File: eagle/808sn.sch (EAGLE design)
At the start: 75 parts, among them IC1 TL072P, IC3 TL072P, Q1 2N3904, Q45 2N3904, Q46 2N3906, Q47 2N3904, Q48 2N3904, Q49 2N3904, U1 POWER

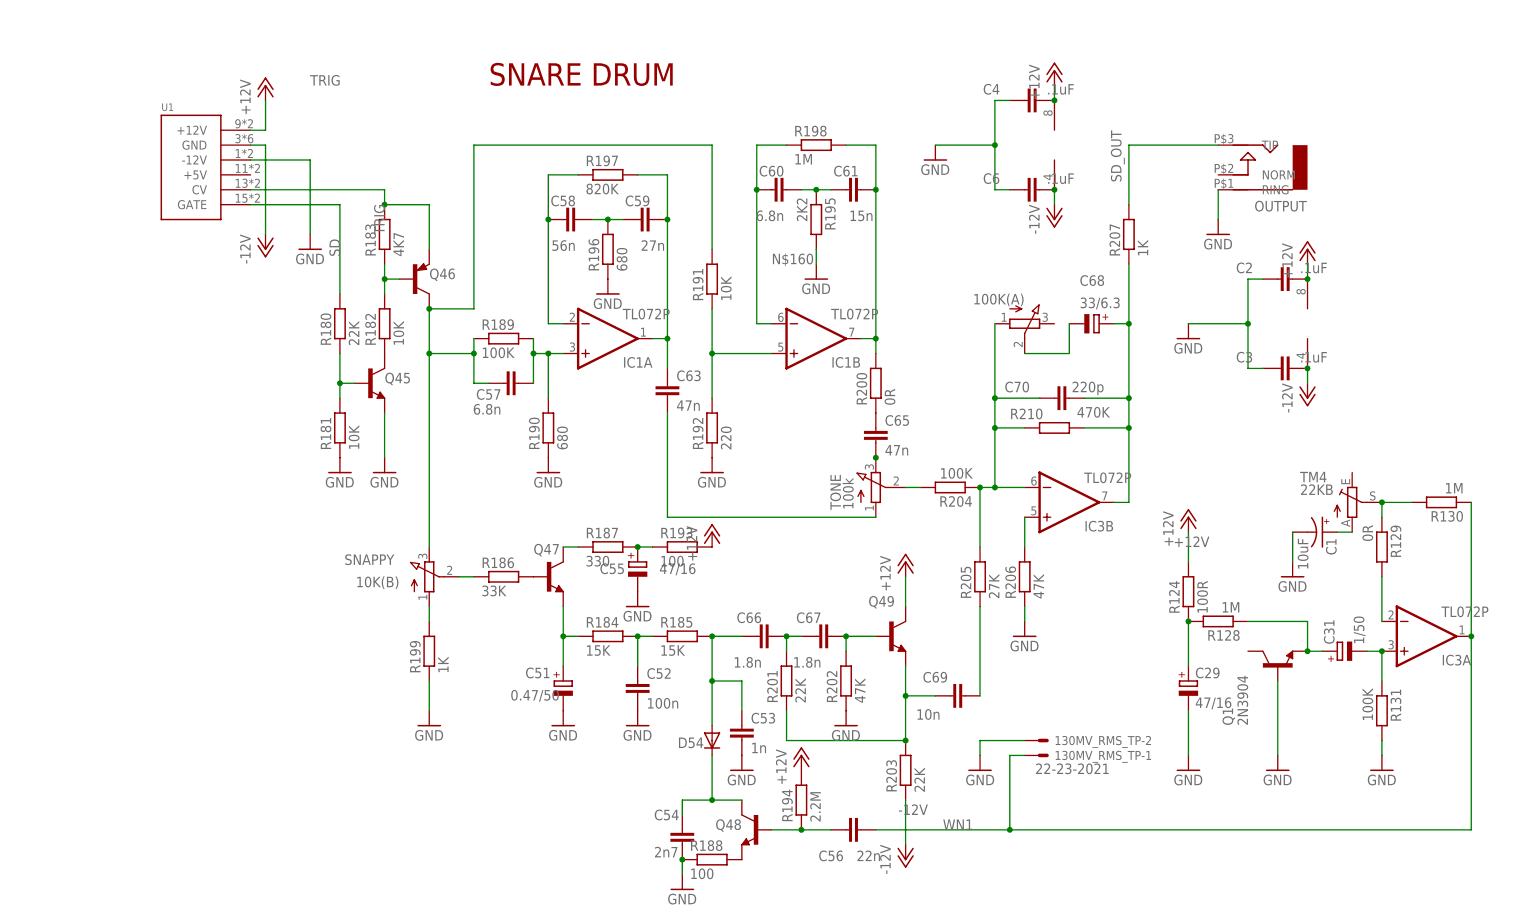
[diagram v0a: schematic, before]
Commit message: 92pct autorouted
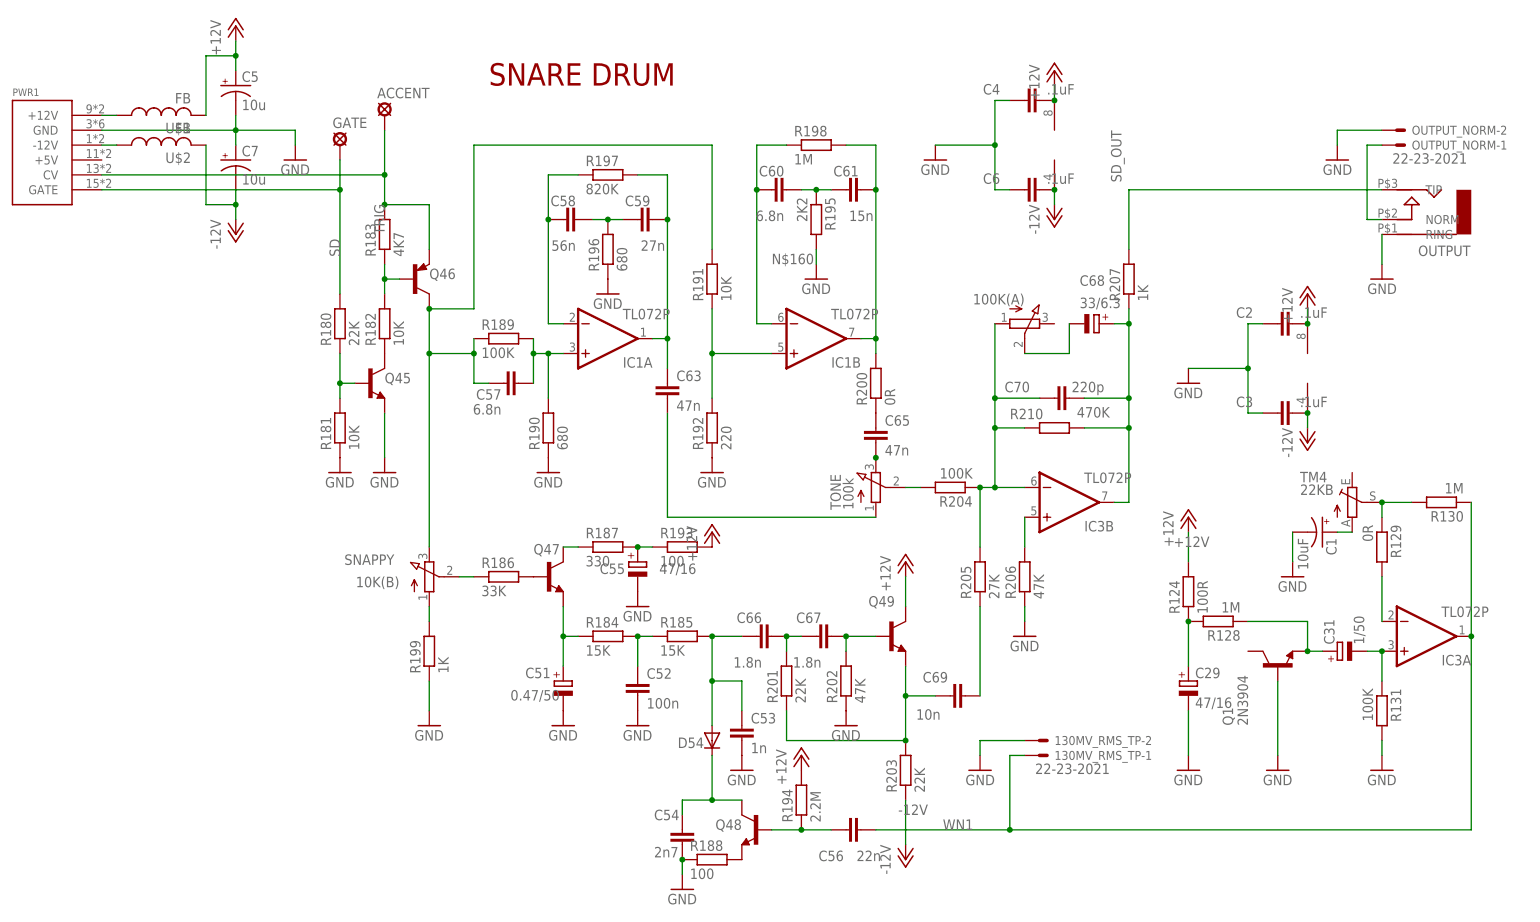
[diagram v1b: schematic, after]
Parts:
- removed U1: POWER, eurorack:POWER
- added ACCENT, GATE: LSP10, solpad:LSP10
- added C5, C7: 10u, rcl:CPOL-USB45181A
- added OUTPUT_NORM: 22-23-2021, con-molex:22-23-2021
- added PWR1: POWER, eurorack:POWER
- added U$1, U$2: FB, adafruit:FB
- R187, R193, R195, R196, R201, R205: device TR808clone:R-EU_0207/5V -> TR808clone:R-EU_0207/7
- R194, R203, R207: device TR808clone:R-EU_0207/5V -> TR808clone:R-EU_0309/10
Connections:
- new net N$10: PWR1.+12V, U$1.1
- new net N$2: OUTPUT.NORM, OUTPUT_NORM-1.S
- new net N$37: PWR1.-12V, U$2.1
- net +12V: now also C5.+, U$1.2; no longer U1.+12V
- net -12V: now also C7.-, U$2.2; no longer U1.GND
- net GND: now also OUTPUT_NORM-2.S; no longer U1.-12V
- net N$26: now also C5.-, C7.+, PWR1.GND
- net SD: now also GATE.MP, PWR1.GATE; no longer U1.GATE
- net TRIG: now also ACCENT.MP, PWR1.CV; no longer U1.CV
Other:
- moved on the sheet: C2, C3, OUTPUT, R207

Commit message: board started over
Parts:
- C52: device TR808clone:C-EU075-032X103 -> TR808clone:C-EU050-045X075
- C6: device TR808clone:C-EU025-025X050 -> TR808clone:C-EU050-025X075
- C69: device TR808clone:C-EU3.5MM_PITCH -> TR808clone:C-EU075-042X103
- R194, R203: device TR808clone:R-EU_0309/10 -> TR808clone:R-EU_0207/7
- R204: device TR808clone:R-EU_0207/5V -> TR808clone:R-EU_0207/7
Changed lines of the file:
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@@
 <part name="R184" library="TR808clone" deviceset="R-EU_" device="0207/5V" value="15K"/>
 <part name="R185" library="TR808clone" deviceset="R-EU_" device="0207/5V" value="15K"/>
-<part name="C52" library="TR808clone" deviceset="C-EU" device="075-032X103" value="100n"/>
+<part name="C52" library="TR808clone" deviceset="C-EU" device="050-045X075" value="100n"/>
 <part name="C55" library="TR808clone" deviceset="CPOL-EU" device="E2-5" value="47/16"/>
 <part name="C51" library="TR808clone" deviceset="CPOL-EU" device="E2-5" value="0.47/50"/>
@@
 <part name="GND13" library="supply1" deviceset="GND" device=""/>
 <part name="GND14" library="supply1" deviceset="GND" device=""/>
-<part name="R203" library="TR808clone" deviceset="R-EU_" device="0309/10" value="22K"/>
+<part name="R203" library="TR808clone" deviceset="R-EU_" device="0207/7" value="22K"/>
 <part name="Q48" library="808_lt" deviceset="2N3904" device=""/>
 <part name="C54" library="TR808clone" deviceset="C-EU" device="3.5MM_PITCH" value="2n7"/>
 <part name="R188" library="TR808clone" deviceset="R-EU_" device="0207/5V" value="100"/>
-<part name="R194" library="TR808clone" deviceset="R-EU_" device="0309/10" value="2.2M"/>
+<part name="R194" library="TR808clone" deviceset="R-EU_" device="0207/7" value="2.2M"/>
 <part name="C56" library="TR808clone" deviceset="C-EU" device="4MM_PITCH" value="22n"/>
 <part name="GND58" library="supply1" deviceset="GND" device=""/>
-<part name="C69" library="TR808clone" deviceset="C-EU" device="3.5MM_PITCH" value="10n"/>
-<part name="R204" library="TR808clone" deviceset="R-EU_" device="0207/5V" value="100K"/>
+<part name="C69" library="TR808clone" deviceset="C-EU" device="075-042X103" value="10n"/>
+<part name="R204" library="TR808clone" deviceset="R-EU_" device="0207/7" value="100K"/>
 <part name="R205" library="TR808clone" deviceset="R-EU_" device="0207/7" value="27K"/>
 <part name="R206" library="TR808clone" deviceset="R-EU_" device="0207/5V" value="47K"/>
@@
 <part name="IC1" library="linear" deviceset="TL072" device="P"/>
 <part name="C4" library="TR808clone" deviceset="C-EU" device="025-025X050" value=".1uF"/>
-<part name="C6" library="TR808clone" deviceset="C-EU" device="025-025X050" value=".1uF"/>
+<part name="C6" library="TR808clone" deviceset="C-EU" device="050-025X075" value=".1uF"/>
 <part name="GND15" library="supply1" deviceset="GND" device=""/>
 <part name="R130" library="TR808clone" deviceset="R-EU_" device="0207/7" value="1M"/>

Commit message: 94pct autorouted
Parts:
- R183, R189: device TR808clone:R-EU_0207/5V -> TR808clone:R-EU_0207/2V
- R186: device TR808clone:R-EU_0207/5V -> TR808clone:R-EU_0309/12
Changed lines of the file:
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@@
 <part name="R181" library="TR808clone" deviceset="R-EU_" device="0207/5V" value="10K"/>
 <part name="R182" library="TR808clone" deviceset="R-EU_" device="0207/5V" value="10K"/>
-<part name="R183" library="TR808clone" deviceset="R-EU_" device="0207/5V" value="4K7"/>
+<part name="R183" library="TR808clone" deviceset="R-EU_" device="0207/2V" value="4K7"/>
 <part name="Q45" library="808_lt" deviceset="2N3904" device=""/>
 <part name="Q46" library="808_lt" deviceset="2N3906" device=""/>
@@
 <part name="C59" library="TR808clone" deviceset="C-EU" device="050-024X044" value="27n"/>
 <part name="C57" library="TR808clone" deviceset="C-EU" device="4MM_PITCH" value="6.8n"/>
-<part name="R189" library="TR808clone" deviceset="R-EU_" device="0207/5V" value="100K"/>
+<part name="R189" library="TR808clone" deviceset="R-EU_" device="0207/2V" value="100K"/>
 <part name="R196" library="TR808clone" deviceset="R-EU_" device="0207/7" value="680"/>
 <part name="R197" library="TR808clone" deviceset="R-EU_" device="0207/5V" value="820K"/>
@@
 <part name="R199" library="TR808clone" deviceset="R-EU_" device="0207/5V" value="1K"/>
 <part name="GND9" library="supply1" deviceset="GND" device=""/>
-<part name="R186" library="TR808clone" deviceset="R-EU_" device="0207/5V" value="33K"/>
+<part name="R186" library="TR808clone" deviceset="R-EU_" device="0309/12" value="33K"/>
 <part name="Q47" library="808_lt" deviceset="2N3904" device=""/>
 <part name="R187" library="TR808clone" deviceset="R-EU_" device="0207/7" value="330"/>
